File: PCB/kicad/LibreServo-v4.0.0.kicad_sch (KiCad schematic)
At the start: 104 parts, among them M1 M1, M2 MOSFET_N+P, M3 MOSFET_N+P, M4 FAN3227/4, M5 FAN3227/4, U1 M0G3519QRHBRQ1, U10 AEAT-8800, U2 MPM3610, U3 AP2112, U4 ACS711, U5 ADM2587E, U6 ADM3055E, U7 SLB 9672AU2.0

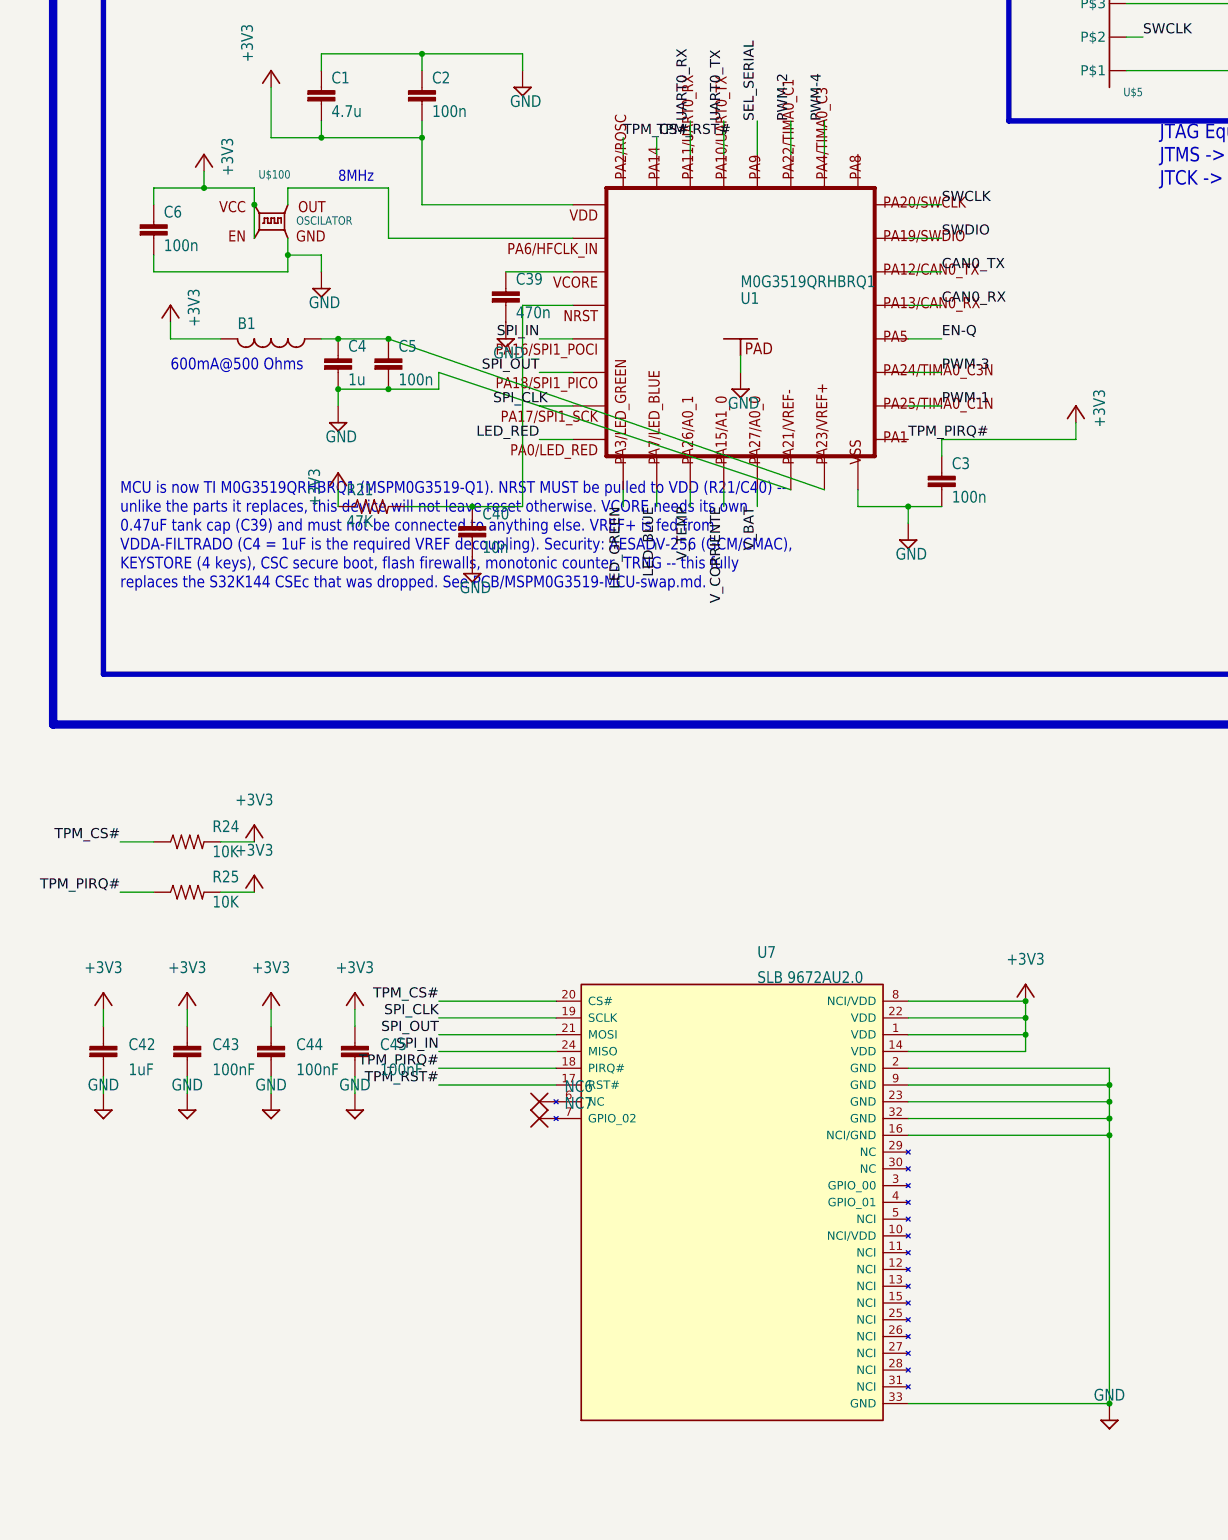
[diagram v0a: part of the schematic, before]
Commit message: feat(pcb): replace the SLB9672 TPM with an OPTIGA Trust M secure element (U7)
The servo needs an independent hardware root of trust, not a TPM stack. U7 was
an Infineon SLB9672 TPM 2.0 -- a 32-pin SPI platform-integrity module built
around PCRs and attestation. It is replaced by an Infineon OPTIGA(TM) Trust M
V3 (SLS 32AIA010ML, ETR -40..+105C, PG-USON-10-2,-4, 3x3mm), a 10-pin I2C key
vault with a crypto engine.

This is NOT a like-for-like substitution and the schematic no longer pretends
otherwise: different device class, different bus, different pin count. The SPI
interface and all six TPM-specific nets are gone.

Schematic changes (tools/swap_slb9672_for_optiga.py, committed so the edit is
reproducible and auditable rather than an untraceable hand pass):
- Deleted the SLB9672_TPM lib_symbol, the U7 instance, and its 16 wires.
- Deleted the six TPM-side label stubs. The SPI_CLK/SPI_IN/SPI_OUT nets
  themselves survive untouched -- they are shared with other devices; only the
  TPM's tap on them is removed.
- Renamed the surviving MCU-side labels so the sheet stops claiming a TPM
  exists: TPM_RST# -> SE_RST, TPM_CS# -> SPARE_PA2, TPM_PIRQ# -> SPARE_PIRQ.
  The last two mark MCU pins the TPM removal genuinely freed.
- Added U7 (Trust M), R30/R31 10k I2C pull-ups, C43 100n decoupling, and
  no-connect flags on the five NC contacts. Circuit per REFERENCES.md [45]
  p.12 Sec.3 Figure 2; the NC contacts must be left floating per [45] p.17
  Table 6, so they are flagged, never tied to a rail.
- Removed two NC_MARKER instances (NC6, NC7) left orphaned on the old TPM's
  unused pins.

New project-owned symbol library LibreServo-v4.0.0.kicad_sym (distinct from
the EAGLE import) holding the Trust M, plus its footprint copied unchanged
from the sister Open-Secure-ESC repo, and both registered in sym-lib-table.
The symbol's Description was rewritten for this board -- the copied text
described the ESC's S32K144/CSEc split and designator U2, which is wrong here.

KNOWN INCOMP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
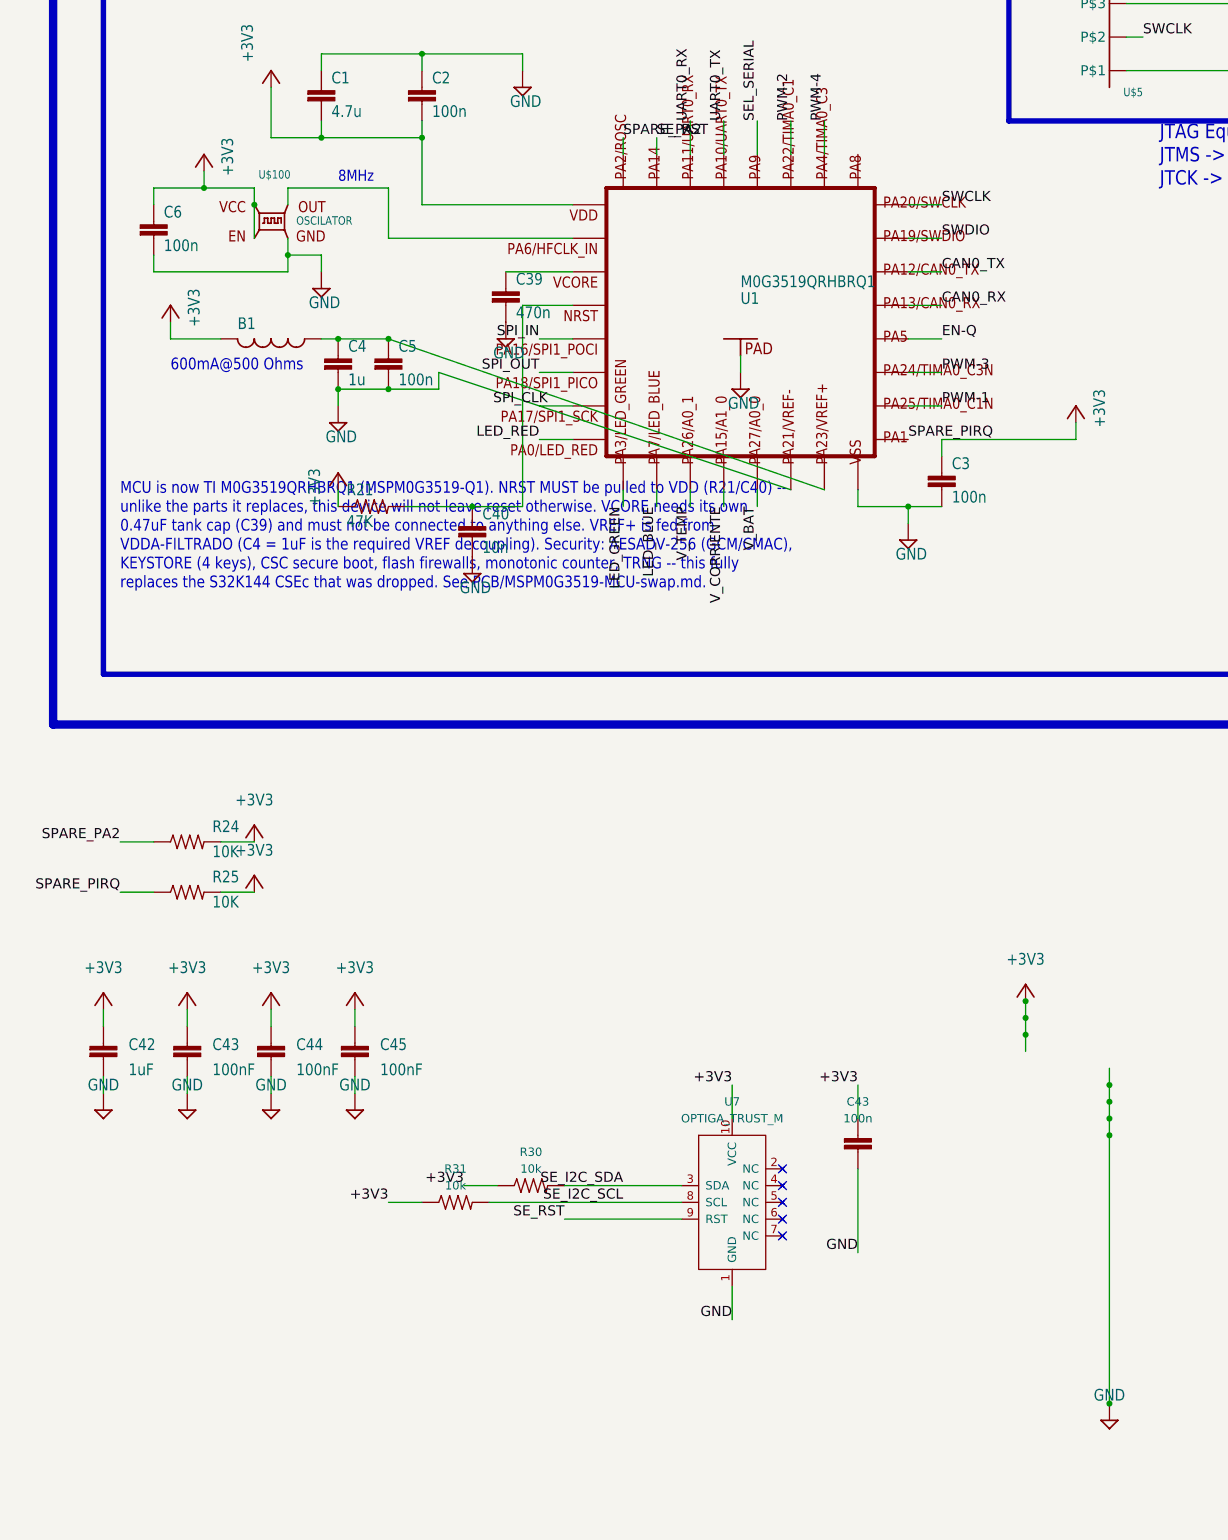
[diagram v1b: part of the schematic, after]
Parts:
- removed NC6, NC7: (no value), symbol LibreServo-v4.0.0-eagle-import:NC_MARKER
- removed U7: SLB 9672AU2.0, Package_DFN_QFN:QFN-32-1EP_5x5mm_P0.5mm_EP3.6x3.6mm, symbol LibreServo-v4.0.0-eagle-import:SLB9672_TPM
- added C43: 100n, LibreServo-v4.0.0:0402, symbol LibreServo-v4.0.0-eagle-import:C-EU0402
- added R30, R31: 10k, LibreServo-v4.0.0:0402, symbol LibreServo-v4.0.0-eagle-import:R-US0402
- added U7: OPTIGA_TRUST_M, LibreServo-v4.0.0:Infineon_PG-USON-10-2-4_3x3mm_P0.5mm_EP1.7x2.5mm, symbol LibreServo-v4.0.0:OPTIGA_TRUST_M
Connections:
- net +3V3: now also C43.1, R30.1, R31.1, U7.10 (VCC)
- net GND: now also C43.2, U7.1 (GND)
- net TPM_CS# renamed SPARE_PA2
- net TPM_PIRQ# renamed SPARE_PIRQ
- net TPM_RST# renamed SE_RST
- net SE_RST: now also U7.9 (RST)
- new net SE_I2C_SCL: R31.2, U7.8 (SCL)
- new net SE_I2C_SDA: R30.2, U7.3 (SDA)
- no-connect marks 0 -> 5

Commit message: Resolve TODO items 1-4: REFERENCES.md intake, MCU pin/part fixes, secure element wiring, security protocol decisions
TODO §1 (Governance & Documentation):
- Complete the REFERENCES.md intake (1.4a-c): add IEEE entries [46]-[52] for
  the MSPM0G351x-Q1 datasheet, both isolated transceiver datasheets, and the
  TI MSPM0 application notes, each read directly from the local PDFs with
  verified section/page citations. Found and recorded that the errata doc
  slaz742g.pdf does not apply to the current MCU die (wrong family).
- Audit README.md for uncited claims (1.6): fixed an unsourced "9Mbps" bus
  speed claim that didn't match either transceiver's real datasheet figures,
  and marked WSD3069DN56/AEAT-8800/ACS711/board-voltage claims UNVERIFIED
  pending datasheet intake.

TODO §3 (MCU Subsystem):
- 3.1: Resolved the blocking I2C pin-pair lookup by re-extracting Table 6-2
  with a column-preserving PDF tool. PA1 (I2C0_SCL) and PA8 (I2C0_SDA) are
  the only I2C-capable pins among the four TPM-era spares.
- 3.2: Reconciled a real MCU part-number mismatch -- U1's placed symbol had
  drifted to MSPM0G3519 (512KB) while README/title-block/swap-doc all
  intended MSPM0G3518 (256KB). Renamed the symbol and fixed Value/Description
  in both the schematic and the symbol library.
- 3.3: Repurposed PA1 as SE_I2C_SCL and formally retired PA2 (no I2C
  capability); set their stale TPM-era pull-ups (R24, R25) to do-not-populate.

TODO §4 (Trust/Security Subsystem):
- 4.3: Wired SE_I2C_SDA/SE_I2C_SCL from the secure element through to the
  MCU pins resolved in 3.1, using pin-coordinate-verified net labels.
- 4.4-4.9: Recorded design decisions for Shielded Connection/platform binding
  secret, anti-replay framing, MAC-failure fail-behaviour, where per-frame
  authentication runs, key lifecycle/revocation, and ECC curve selection in
  a new PCB/servo-bus-security-protocol.md, each grounded in the Trust M and
  MCU datasheets and explicitly flagged as judgment calls where no standard
 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
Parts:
- R24, R25: now not fitted
- U1: value M0G3519QRHBRQ1 -> M0G3518QRHBRQ1; symbol LibreServo-v4.0.0-eagle-import:MSPM0G3519 -> LibreServo-v4.0.0-eagle-import:MSPM0G3518
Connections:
- net SPARE_PIRQ is gone; now on net SE_I2C_SCL: R25.1, U1.2 (PA1)
- net SE_I2C_SDA: now also U1.12 (PA8)
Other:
- note added: "MCU is now TI M0G3518QRHBRQ1 (MSPM0G3518-Q1). NRST MUST be pulled to VDD (R21/C40) -- unlike the parts it replaces, this device will not leave reset otherwise. VCORE needs its own 0.47uF tank cap (C39) and must not be connected to anything else. VREF+ is fed from VDDA-FILTRADO (C4 = 1uF is the required VREF decoupling). Security: AESADV-256 (GCM/CMAC), KEYSTORE (4 keys), CSC secure boot, flash fi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"
- note added: "MSPM0G3518-Q1 (VQFN-32 RHB, 5x5mm) @ 80MHz Cortex-M0+, 256KB/128KB, AEC-Q100 Grade 1"
- note removed: "MCU is now TI M0G3519QRHBRQ1 (MSPM0G3519-Q1). NRST MUST be pulled to VDD (R21/C40) -- unlike the parts it replaces, this device will not leave reset otherwise. VCORE needs its own 0.47uF tank cap (C39) and must not be connected to anything else. VREF+ is fed from VDDA-FILTRADO (C4 = 1uF is the required VREF decoupling). Security: AESADV-256 (GCM/CMAC), KEYSTORE (4 keys), CSC secure boot, flash fi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"
- note removed: "MSPM0G3519-Q1 (VQFN-32 RHB, 5x5mm) @ 80MHz Cortex-M0+, 512KB/128KB, AEC-Q100 Grade 1"
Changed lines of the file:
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@@
 		)
 	)
-	(text "MCU is now TI M0G3519QRHBRQ1 (MSPM0G3519-Q1). NRST MUST be pulled to VDD (R21/C40) --\nunlike the parts it replaces, this device will not leave reset otherwise. VCORE needs its own\n0.47uF tank cap (C39) and must not be connected to anything else. VREF+ is fed from\nVDDA-FILTRADO (C4 = 1uF is the required VREF decoupling). Security: AESADV-256 (GCM/CMAC),\nKEYSTORE (4 keys), CSC secure boot, flash firewalls, monotonic counter, TRNG -- this fully\nreplaces the S32K144 CSEc that was dropped. See PCB/MSPM0G3519-MCU-swap.md."
+	(text "MCU is now TI M0G3518QRHBRQ1 (MSPM0G3518-Q1). NRST MUST be pulled to VDD (R21/C40) --\nunlike the parts it replaces, this device will not leave reset otherwise. VCORE needs its own\n0.47uF tank cap (C39) and must not be connected to anything else. VREF+ is fed from\nVDDA-FILTRADO (C4 = 1uF is the required VREF decoupling). Security: AESADV-256 (GCM/CMAC),\nKEYSTORE (4 keys), CSC secure boot, flash firewalls, monotonic counter, TRNG -- this fully\nreplaces the S32K144 CSEc that was dropped. SE_I2C_SDA/SE_I2C_SCL now wired to PA8/PA1 -- see\nTODO.md 3.1/4.3. See PCB/MSPM0G3518-MCU-swap.md."
 		(exclude_from_sim no)
 		(at 27.94 317.5 0)
@@
 		)
 	)
-	(text "MSPM0G3519-Q1 (VQFN-32 RHB, 5x5mm) @ 80MHz Cortex-M0+, 512KB/128KB, AEC-Q100 Grade 1"
+	(text "MSPM0G3518-Q1 (VQFN-32 RHB, 5x5mm) @ 80MHz Cortex-M0+, 256KB/128KB, AEC-Q100 Grade 1"
 		(exclude_from_sim no)
 		(at 27.94 220.98 0)
@@
 	)
 	(symbol
-		(lib_id "LibreServo-v4.0.0-eagle-import:MSPM0G3519")
+		(lib_id "LibreServo-v4.0.0-eagle-import:MSPM0G3518")
 		(at 121.92 276.86 0)
 		(unit 1)
@@
 			)
 		)
-		(property "Value" "M0G3519QRHBRQ1"
+		(property "Value" "M0G3518QRHBRQ1"
 			(at 121.92 271.78 0)
 			(effects
@@
 		(in_bom yes)
 		(on_board yes)
-		(dnp no)
+		(dnp yes)
 		(property "Reference" "R24"
 			(at 41.910000000000004 354.33000000000004 0)
@@
 		(in_bom yes)
 		(on_board yes)
-		(dnp no)
+		(dnp yes)
 		(property "Reference" "R25"
 			(at 41.910000000000004 361.95000000000005 0)
@@
 		)
 	)
-	(label "SPARE_PIRQ"
+	(label "SE_I2C_SCL"
 		(at 27.94 363.22 0)
 		(effects
@@
 		)
 	)
-	(label "SPARE_PIRQ"
+	(label "SE_I2C_SCL"
 		(at 147.32 294.64 0)
 		(effects
 			(font
+				(size 1.5291 1.5291)
+			)
+			(justify left bottom)
+		)
+	)
+	(label "SE_I2C_SDA"
+		(at 139.7 251.46 0)
+		(effects
+			(font
